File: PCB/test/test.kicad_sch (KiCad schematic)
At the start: 63 parts, among them U1 STM32WBxx_QFN48, U2 USBLC6-2SC6, U3 LD3985M33R, U4 SFH_7072, X1 NX2016_32MHz, X2 NX2012_32K768Hz

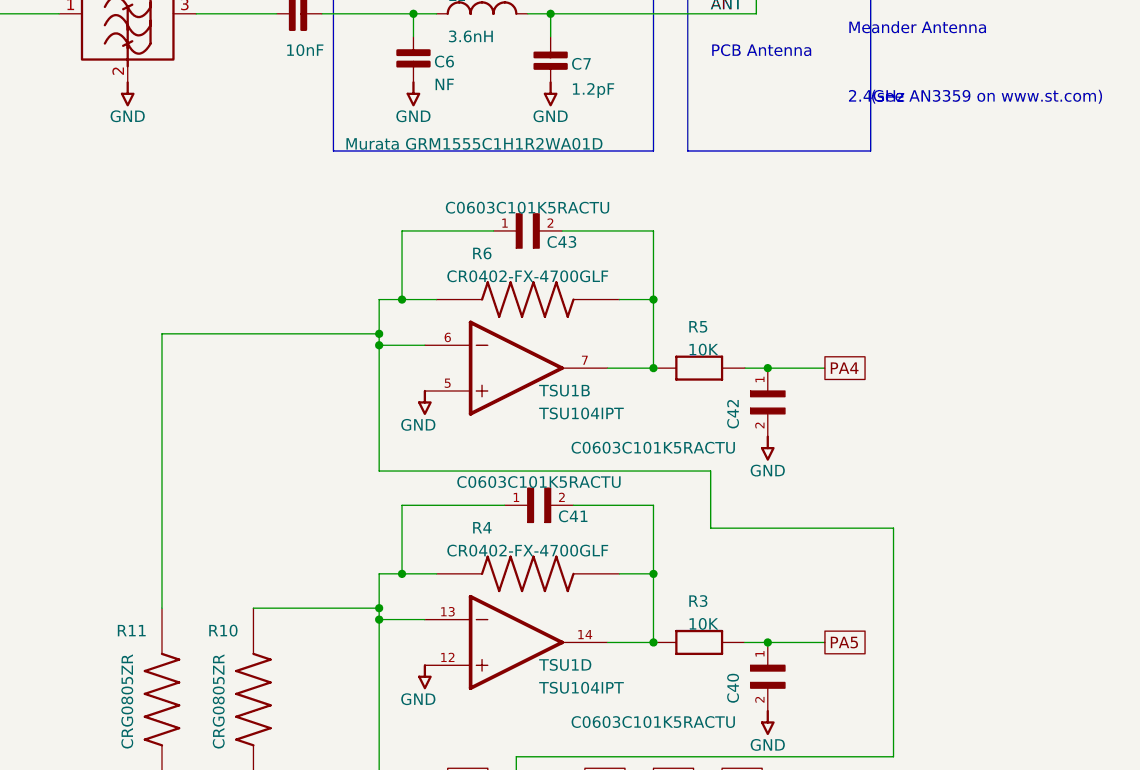
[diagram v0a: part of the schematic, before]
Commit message: ajout alim TSU104
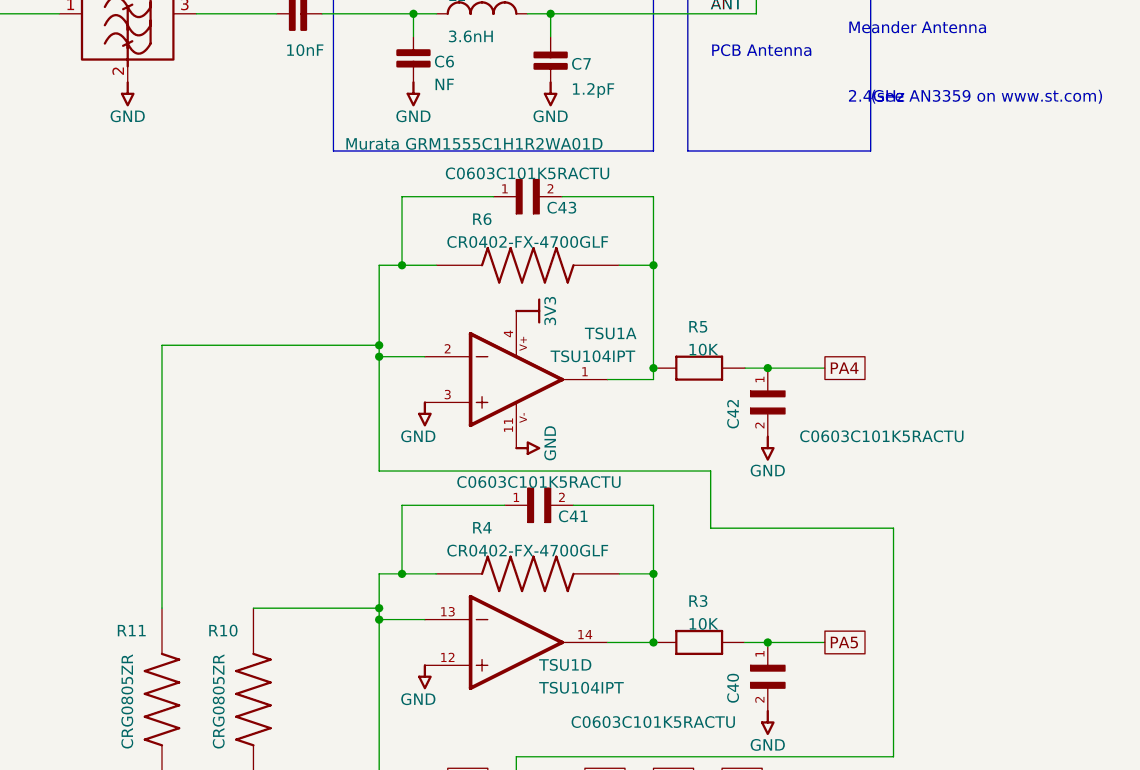
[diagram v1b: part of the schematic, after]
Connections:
- net 3V3: now also TSU1.4
- net GND: now also TSU1.11, TSU1.3; no longer TSU1.5
- net at C43.2, R5.1, R6.2: now also TSU1.1; no longer TSU1.7
- net at C43.1, R11.1, R6.1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: now also TSU1.2; no longer TSU1.6
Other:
- moved on the sheet: C43, R6
